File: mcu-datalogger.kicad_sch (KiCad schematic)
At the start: 25 parts, among them U1 24LC1025, U2 DS1337S+T&R, U3 24LC1025, U4 ATMEGA328-AU, Y1 32.768 KHz, Y2 16MHz

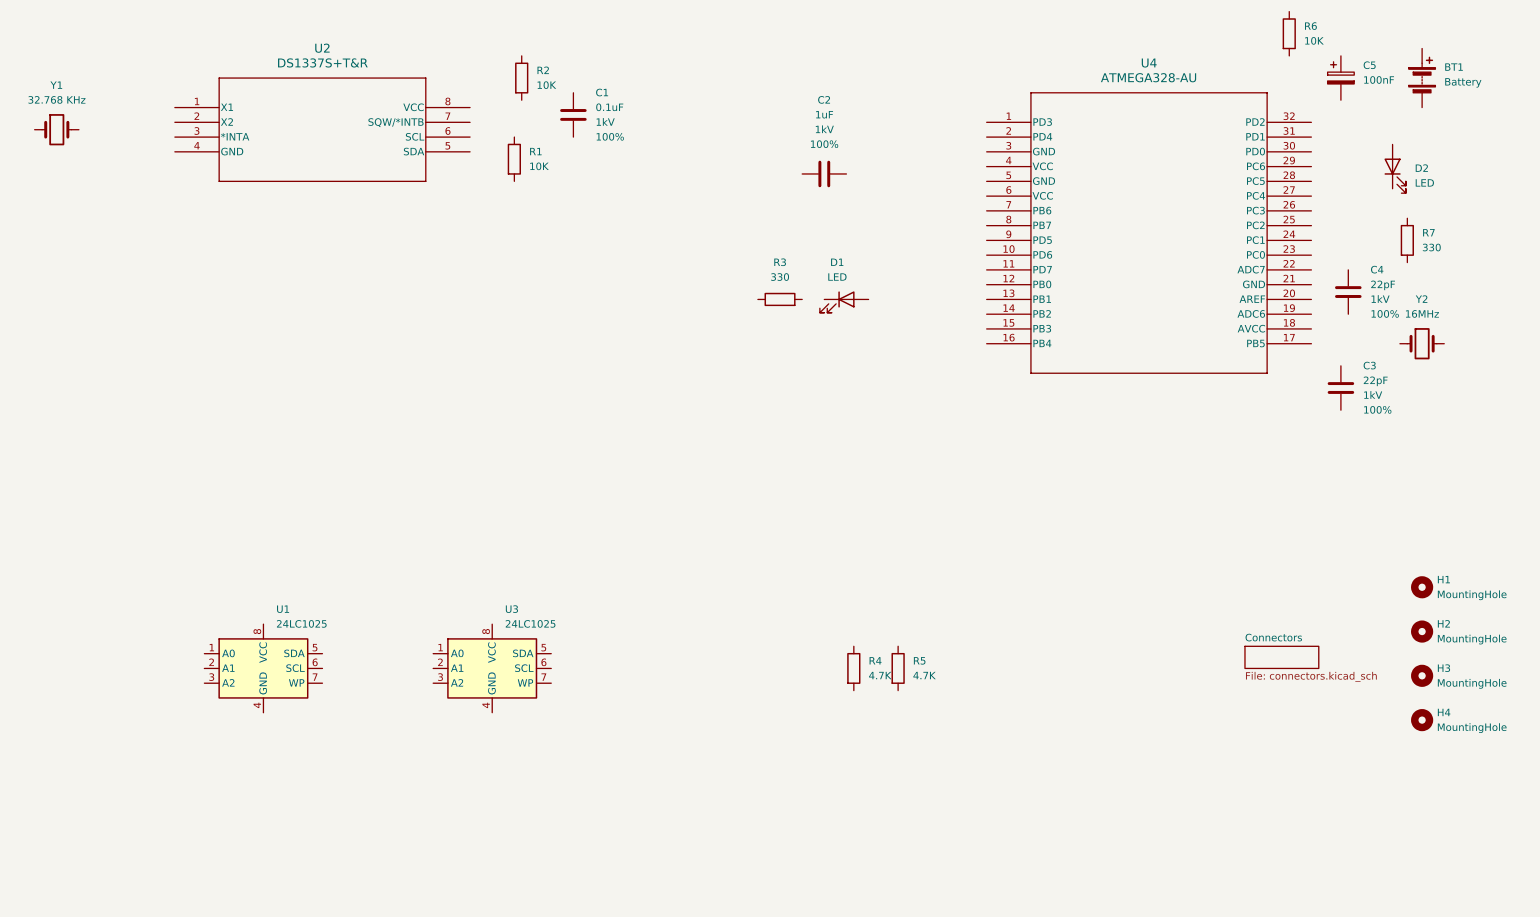
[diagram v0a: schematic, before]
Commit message: Wire main sheet
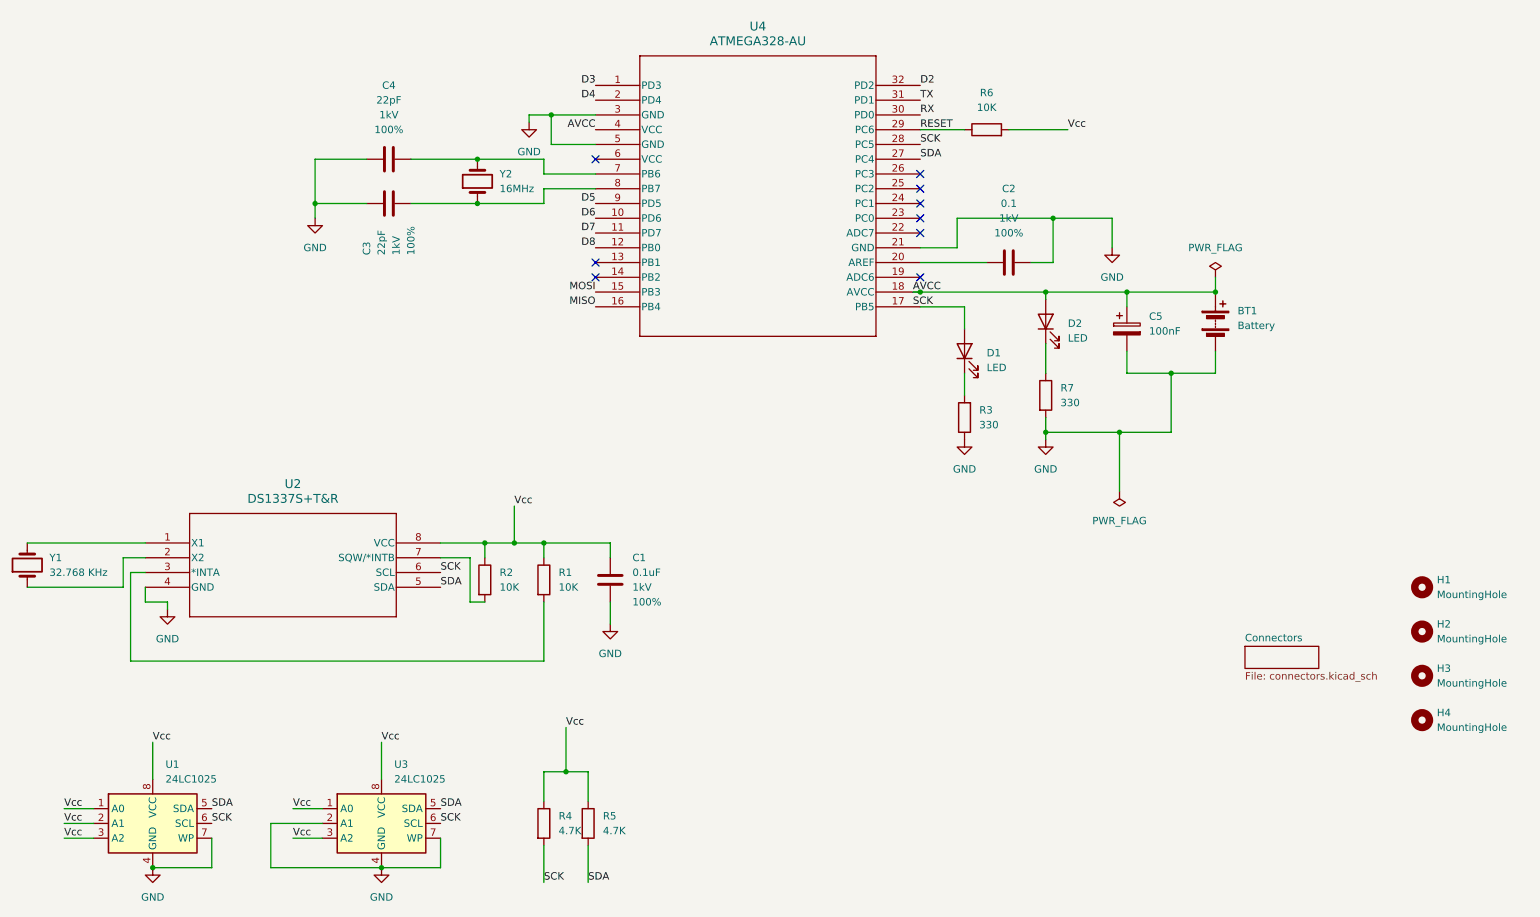
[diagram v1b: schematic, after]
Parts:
- C2: value 1uF -> 0.1
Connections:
- net at Y2.1: now also C3.2, U4.8 (PB7)
- net at Y2.2: now also C4.2, U4.7 (PB6)
- net RESET: now reaches R6.1
- net RESET: now also U4.29 (PC6)
- net Vcc: now reaches R6.2
- net Vcc: now also C1.1, R1.1, R2.1, R4.1, R5.1, U1.1 (A0), U1.2 (A1), U1.3 (A2), U1.8 (VCC), U2.8 (VCC), U3.1 (A0), U3.3 (A2), U3.8 (VCC)
- net at R2.2: now also U2.7 (SQW/*INTB)
- net D3: now reaches U4.1 (PD3)
- net D6: now reaches U4.10 (PD6)
- net D7: now reaches U4.11 (PD7)
- net D8: now reaches U4.12 (PB0)
- net MOSI: now reaches U4.15 (PB3)
- net MISO: now reaches U4.16 (PB4)
- net at U4.17 (PB5): now also D1.2 (A)
- net AVCC: now reaches U4.18 (AVCC)
- net AVCC: now also BT1.1 (+), C5.1, D2.2 (A), U4.4 (VCC)
- net D4: now reaches U4.2 (PD4)
- net at U4.20 (AREF): now also C2.1
- net GND: now reaches U4.21 (GND)
- net GND: now also BT1.2 (-), C1.2, C2.2, C3.1, C4.1, C5.2, R3.1, R7.2, U1.4 (GND), U1.7 (WP), U2.4 (GND), U3.2 (A1), U3.4 (GND), U3.7 (WP), U4.3 (GND), U4.5 (GND)
- net SDA: now reaches U4.27 (PC4)
- net SDA: now also R5.2, U1.5 (SDA), U2.5 (SDA), U3.5 (SDA)
- net SCK: now reaches U4.28 (PC5)
- net SCK: now also R4.2, U1.6 (SCL), U2.6 (SCL), U3.6 (SCL)
- net RX: now reaches U4.30 (PD0)
- net TX: now reaches U4.31 (PD1)
- net D2: now reaches U4.32 (PD2)
- net D5: now reaches U4.9 (PD5)
- net at Y1.1: now also U2.2 (X2)
- net at Y1.2: now also U2.1 (X1)
- net at D2.1 (K): now also R7.1
- net at R1.2: now also U2.3 (*INTA)
- net at R3.2: now also D1.1 (K)
- no-connect marks 0 -> 9
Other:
- moved on the sheet: BT1, C1, C2, C3, C4, C5, D1, D2, R1, R2, R3, R4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
